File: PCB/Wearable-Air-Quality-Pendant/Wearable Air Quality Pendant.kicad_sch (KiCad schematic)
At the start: 46 parts, among them IC1 MCP73832T-2ACI_MC, IC2 ADPL44002AUJZ, IC3 SGP40-D-R4, J1 USB_C_Receptacle_USB2.0_16P, J2 SWD, J3 UART, Q1 SS8550, U1 STM32U083KCUx

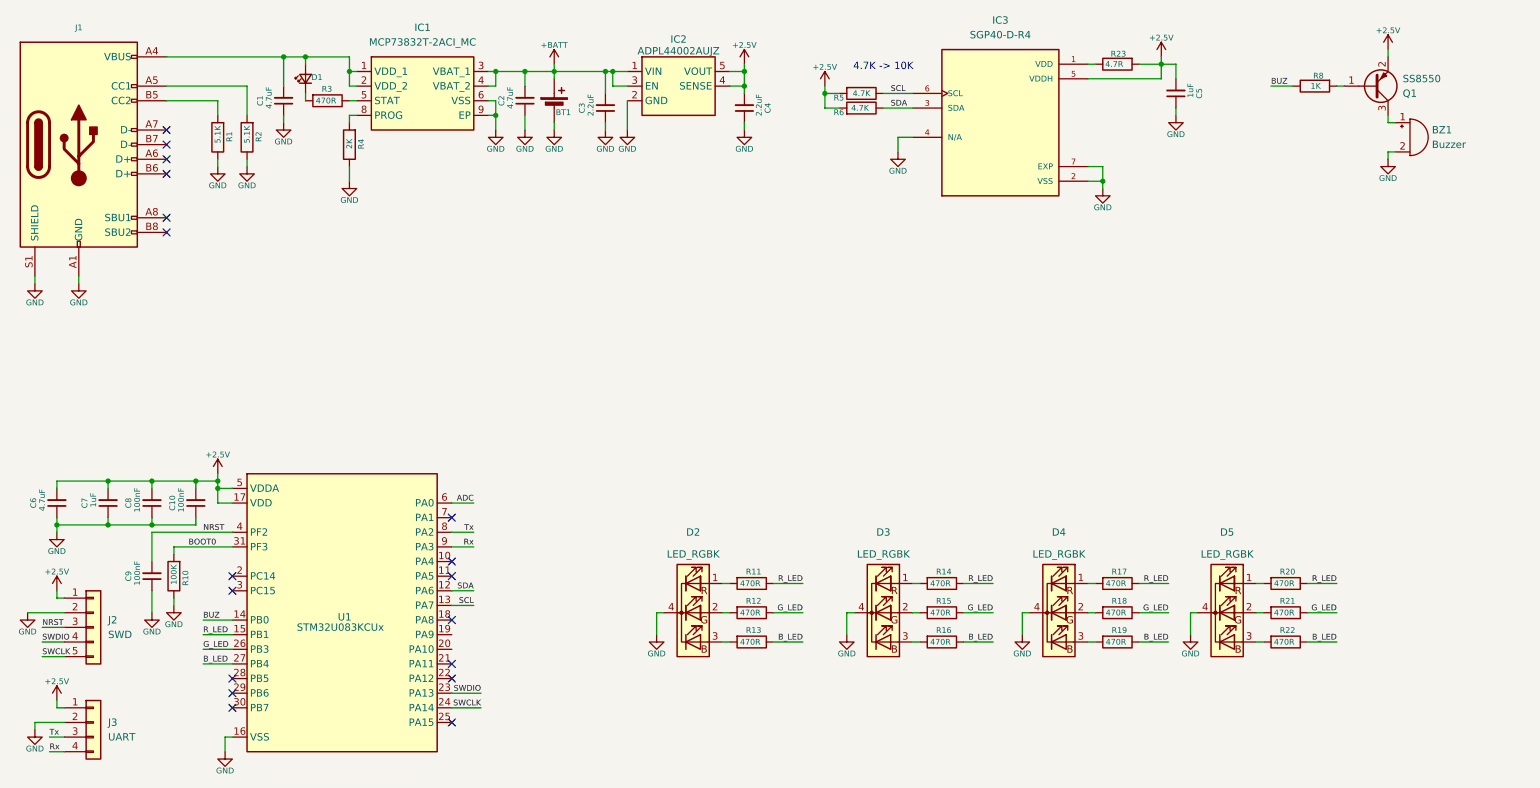
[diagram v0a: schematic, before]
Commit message: Add files via upload
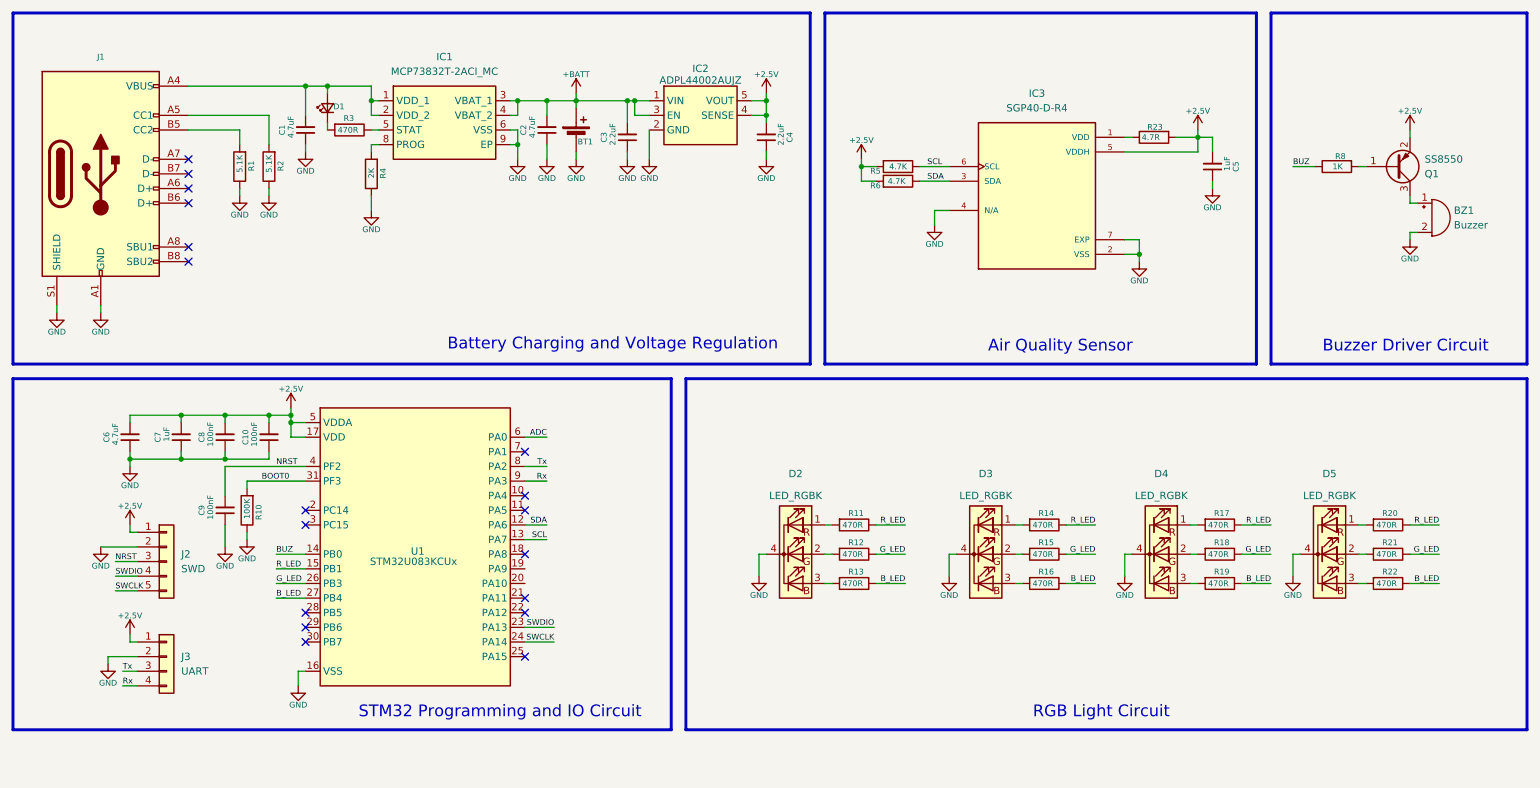
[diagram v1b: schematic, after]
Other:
- note added: "Air Quality Sensor"
- note added: "Battery Charging and Voltage Regulation"
- note added: "Buzzer Driver Circuit"
- note added: "RGB Light Circuit"
- note added: "STM32 Programming and IO Circuit"
- note removed: "4.7K -> 10K"
- moved on the sheet: BT1, BZ1, C1, C10, C2, C3, C4, C5, C6, C7, C8, C9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
